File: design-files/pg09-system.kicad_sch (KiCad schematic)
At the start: 11 parts, among them U101 MC6809E, U102 GAL22V10, U103 74AHCT245, U104 74AHCT245, U105 74AHCT245

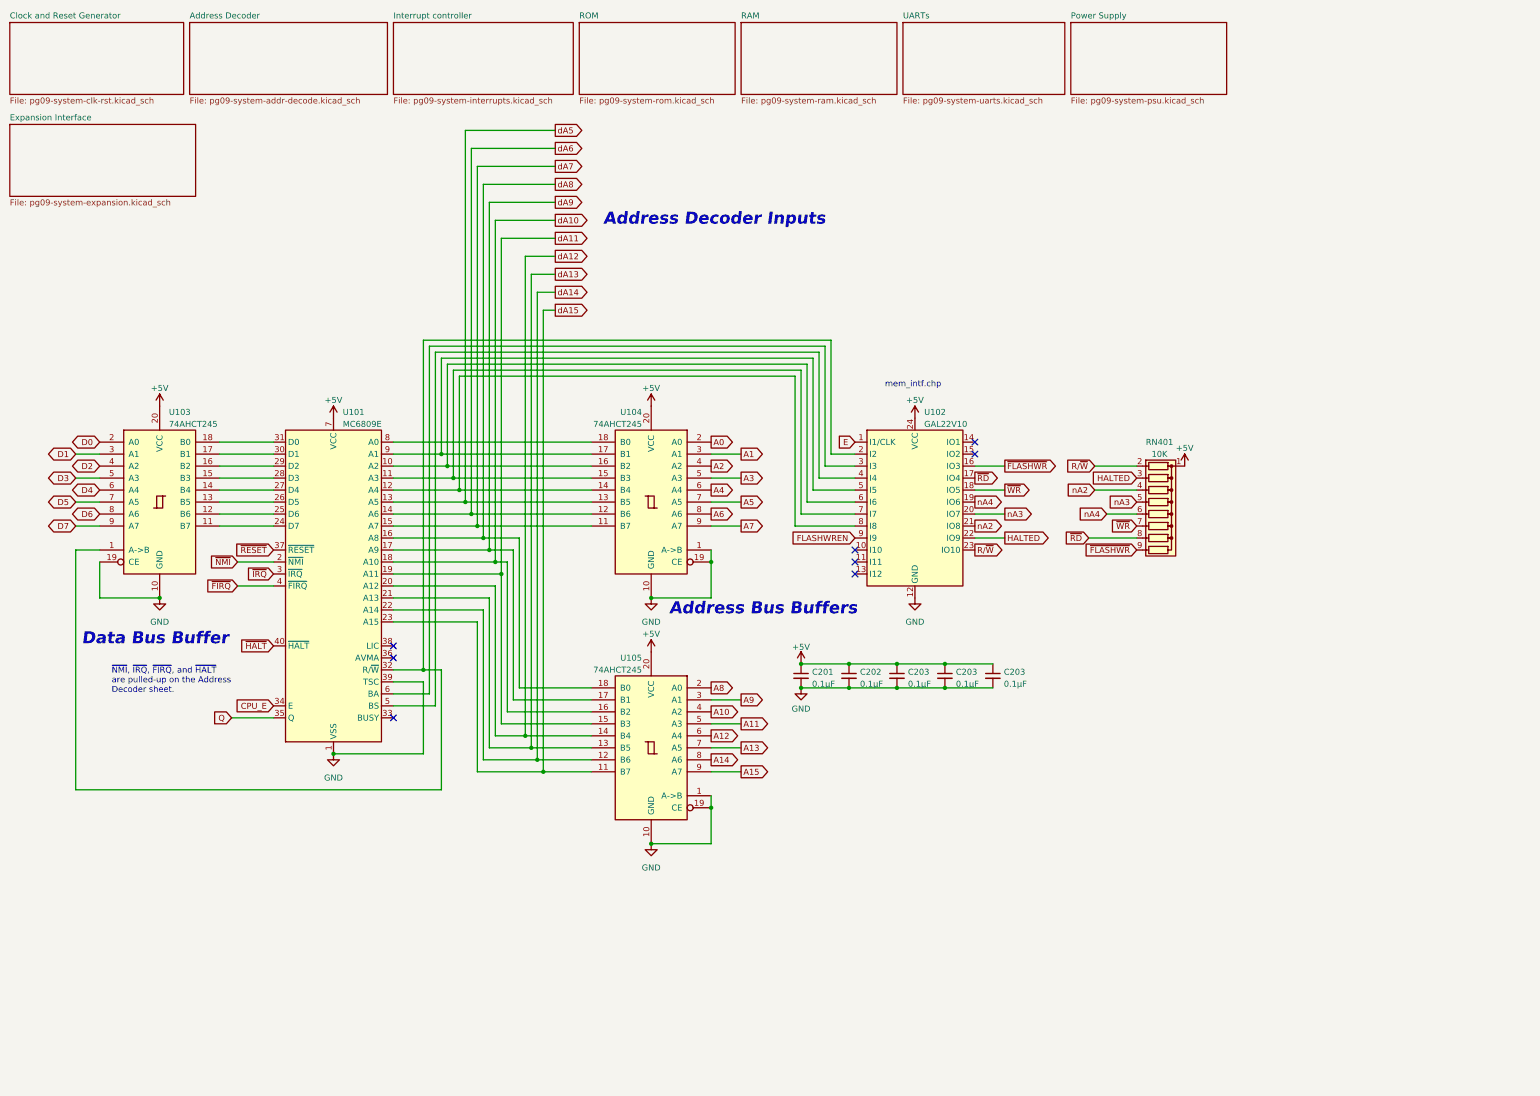
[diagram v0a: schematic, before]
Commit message: Integrate the auto-vectoring interrupt controller.
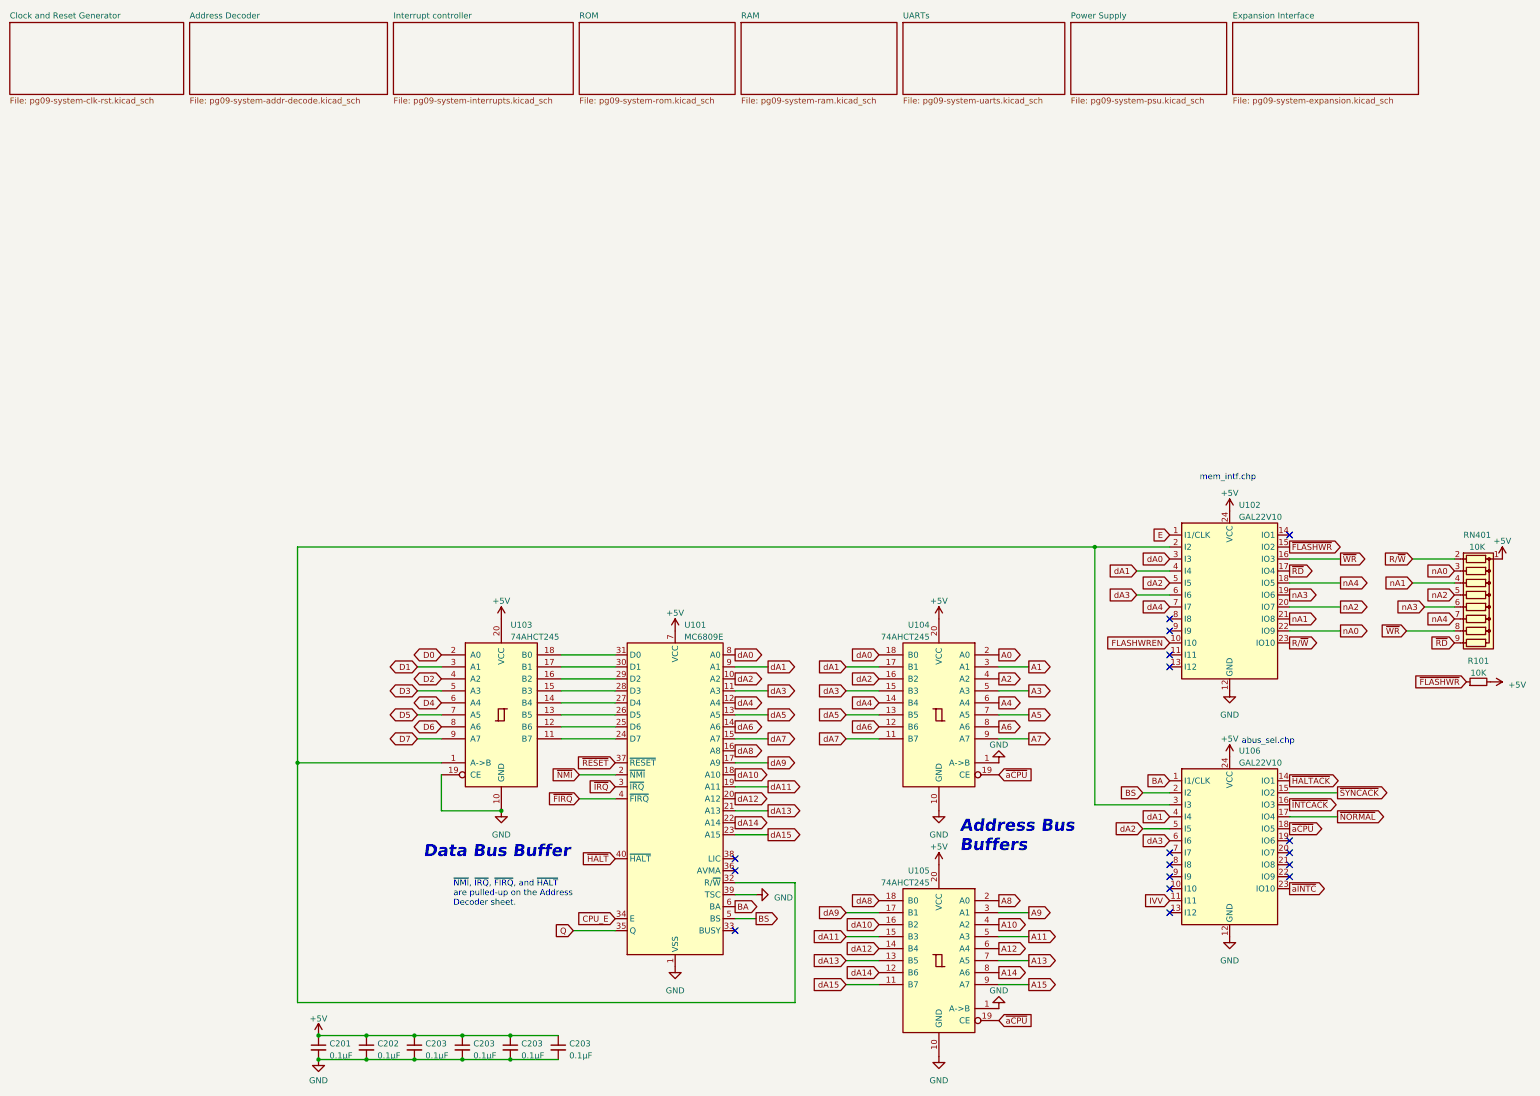
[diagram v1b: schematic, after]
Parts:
- added C203: 0.1µF, Capacitor_THT:C_Disc_D3.8mm_W2.6mm_P2.50mm, symbol Device:C_Small
- added R101: 10K, symbol Device:R_Small
- added U106: GAL22V10, Package_DIP:DIP-24_W7.62mm_Socket, symbol jrt-ICs:GAL22V10
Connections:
- net +5V: now also C203.1, R101.2, U106.24 (VCC)
- net FLASHWREN: now also U102.10 (I10); no longer U102.9 (I9)
- net GND: now also C203.2, U106.12 (GND); no longer U104.19 (CE), U105.19 (CE)
- net nA2: now also RN401.5 (R4), U102.20 (IO7); no longer RN401.4 (R3), U102.21 (IO8)
- net nA3: now also RN401.6 (R5), U102.19 (IO6); no longer RN401.5 (R4), U102.20 (IO7)
- net nA4: now also RN401.7 (R6), U102.18 (IO5); no longer RN401.6 (R5), U102.19 (IO6)
- net ~{FLASHWR}: now also U102.15 (IO2), R101.1; no longer RN401.9 (R8), U102.16 (IO3)
- net ~{RD}: now also RN401.9 (R8); no longer RN401.8 (R7)
- net ~{WR}: now also RN401.8 (R7), U102.16 (IO3); no longer RN401.7 (R6), U102.18 (IO5)
- net dA2: now reaches U101.10 (A2), U104.16 (B2)
- net dA2: now also U102.5 (I5), U106.5 (I5); no longer U102.6 (I6)
- net dA3: now reaches U101.11 (A3), U104.15 (B3)
- net dA3: now also U102.6 (I6), U106.6 (I6); no longer U102.7 (I7)
- net dA4: now reaches U101.12 (A4), U104.14 (B4)
- net dA4: now also U102.7 (I7); no longer U102.8 (I8)
- net at U101.32 (R/~{W}), U102.2 (I2), U103.1 (A->B): now also U106.3 (I3)
- net BS: now reaches U101.5 (BS)
- net BS: now also U106.2 (I2); no longer U102.4 (I4)
- net BA: now reaches U101.6 (BA)
- net BA: now also U106.1 (I1/CLK); no longer U102.3 (I3)
- net dA0: now reaches U101.8 (A0), U104.18 (B0)
- net dA0: now also U102.3 (I3)
- net dA1: now reaches U101.9 (A1), U104.17 (B1)
- net dA1: now also U102.4 (I4), U106.4 (I4); no longer U102.5 (I5)
- net HALTED renamed nA0
- new net IVV: U106.11 (I11)
- new net nA1: RN401.4 (R3), U102.21 (IO8)
- new net ~{HALTACK}: U106.14 (IO1)
- new net ~{INTCACK}: U106.16 (IO3)
- new net ~{NORMAL}: U106.17 (IO4)
- new net ~{SYNCACK}: U106.15 (IO2)
- new net ~{aCPU}: U104.19 (CE), U105.19 (CE), U106.18 (IO5)
- new net ~{aINTC}: U106.23 (IO10)
- no-connect marks 8 -> 17
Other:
- note added: "abus_sel.chp"
- note removed: "Address Decoder Inputs"
- moved on the sheet: C201, C202, C203, RN401, U101, U102, U103, U104, U105
